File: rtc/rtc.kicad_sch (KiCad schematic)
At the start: 16 parts, among them J1 Conn_02x03_Odd_Even, J2 SM04B-SRSS-TB, J3 SM04B-SRSS-TB, J4 SM04B-SRSS-TB, U1 PCF8563, Y1 32.768K12.5PI/MC306

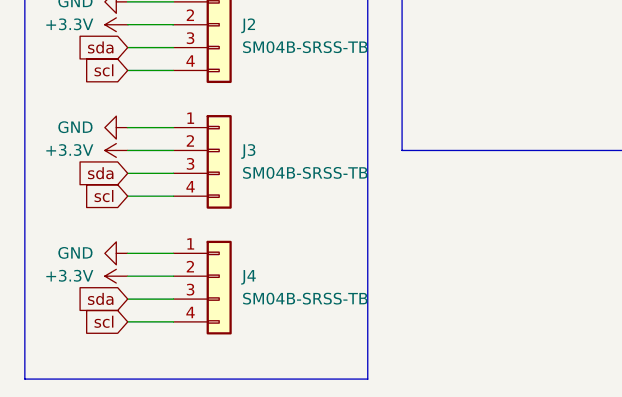
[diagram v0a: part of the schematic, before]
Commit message: rtc_commit
pushed to git properly
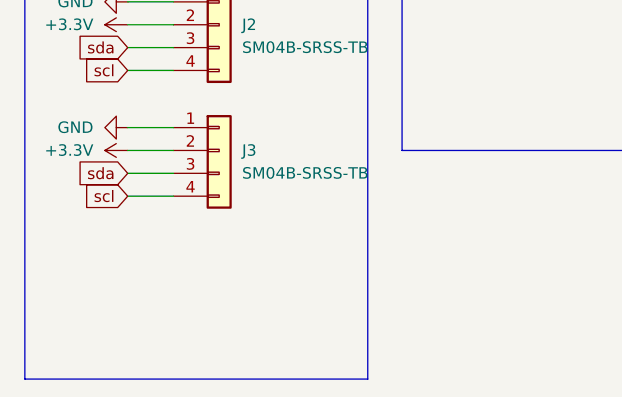
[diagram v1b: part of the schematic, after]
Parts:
- removed J4: SM04B-SRSS-TB, pcb_footprints:SM04BSRSSTB, symbol Connector_Generic:Conn_01x04
